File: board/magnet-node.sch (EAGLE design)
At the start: 36 parts, among them IC1 HTU21D, X1 SMA-142-0701-801/806, X2 SMA-142-0711-821/826

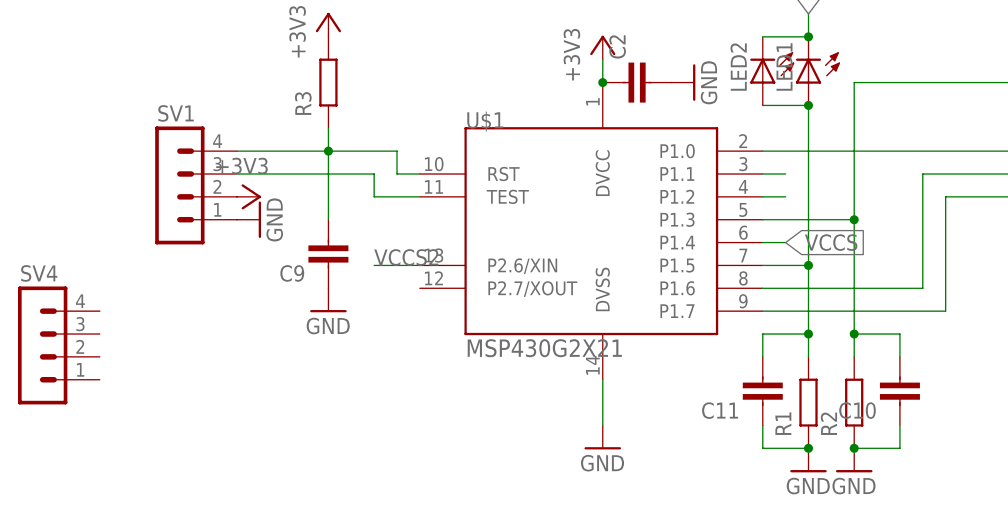
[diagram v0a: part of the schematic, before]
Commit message: small changes
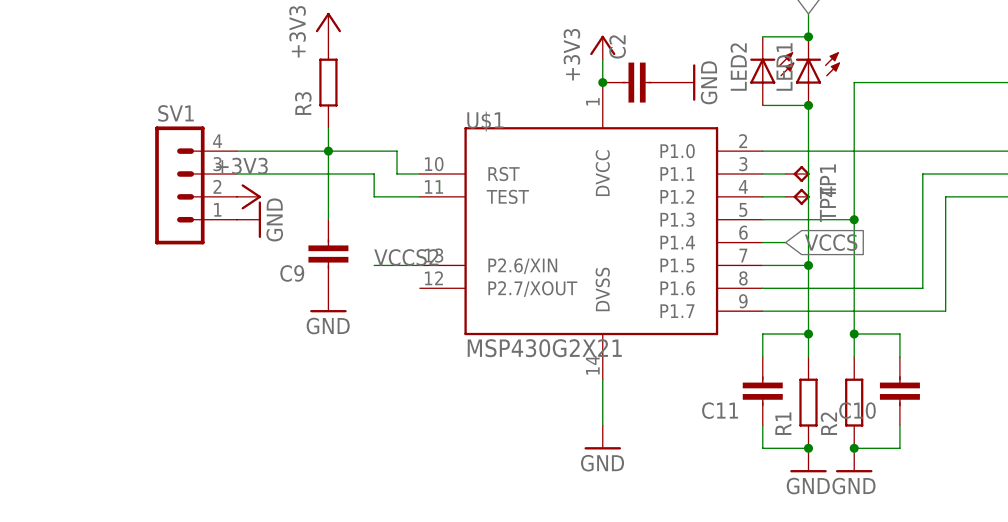
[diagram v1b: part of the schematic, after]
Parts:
- removed SV4: (no value), Mine:MA04-1E
- added TP1, TP4: TPTP14SQ, testpad:TPTP14SQ
- L5: device passives-7351:INDUCTOR0402-N -> passives-7351:INDUCTOR0603-N
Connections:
- net N$11: now also TP1.TP
- net N$14: now also TP4.TP
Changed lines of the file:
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@@
 <part name="U$3" library="Mine" deviceset="LMT85" device=""/>
 <part name="IC1" library="Mine" deviceset="HTU21D" device=""/>
-<part name="SV4" library="Mine" deviceset="MA04-1" device="E"/>
 <part name="GND17" library="supply1" deviceset="GND" device=""/>
 <part name="C12" library="passives-7351" deviceset="CAPACITOR" device="0603-N"/>
@@
 <part name="L3" library="passives-7351" deviceset="INDUCTOR" device="0402-N" value="3.6n"/>
 <part name="L4" library="passives-7351" deviceset="INDUCTOR" device="0402-N" value="3.6n"/>
-<part name="L5" library="passives-7351" deviceset="INDUCTOR" device="0402-N" value="120n"/>
+<part name="L5" library="passives-7351" deviceset="INDUCTOR" device="0603-N" value="120n"/>
+<part name="TP4" library="testpad" deviceset="TP" device="TP14SQ"/>
+<part name="TP1" library="testpad" deviceset="TP" device="TP14SQ"/>
 </parts>
 <sheets>
@@
 <instance part="U$3" gate="G$1" x="134.62" y="99.06"/>
 <instance part="IC1" gate="G$1" x="48.26" y="104.14"/>
-<instance part="SV4" gate="1" x="-17.78" y="30.48"/>
 <instance part="GND17" gate="1" x="53.34" y="88.9"/>
 <instance part="C12" gate="G$1" x="58.42" y="119.38" rot="R90"/>
@@
 <instance part="L4" gate="G$1" x="162.56" y="58.42" rot="R90"/>
 <instance part="L5" gate="G$1" x="162.56" y="73.66" rot="R90"/>
+<instance part="TP4" gate="G$1" x="68.58" y="45.72" rot="R270"/>
+<instance part="TP1" gate="G$1" x="68.58" y="48.26" rot="R270"/>
 </instances>
 <busses>
@@
 <pinref part="U$1" gate="G$1" pin="P1.1"/>
 <wire x1="63.5" y1="48.26" x2="66.04" y2="48.26" width="0.1524" layer="91"/>
+<pinref part="TP1" gate="G$1" pin="TP"/>
 </segment>
 </net>
@@
 <pinref part="U$1" gate="G$1" pin="P1.2"/>
 <wire x1="66.04" y1="45.72" x2="63.5" y2="45.72" width="0.1524" layer="91"/>
-</segment>
-</net>
+<pinref part="TP4" gate="G$1" pin="TP"/>
+</segment>
+</net>
